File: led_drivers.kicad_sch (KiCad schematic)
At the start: 23 parts, among them IC1 SamacSys_Parts_HT16K33-28SOP, IC2 SamacSys_Parts_HT16K33-28SOP, SW1 SW_Omron_B3FS, SW2 SW_Omron_B3FS, SW3 SW_Omron_B3FS, SW4 SW_Omron_B3FS

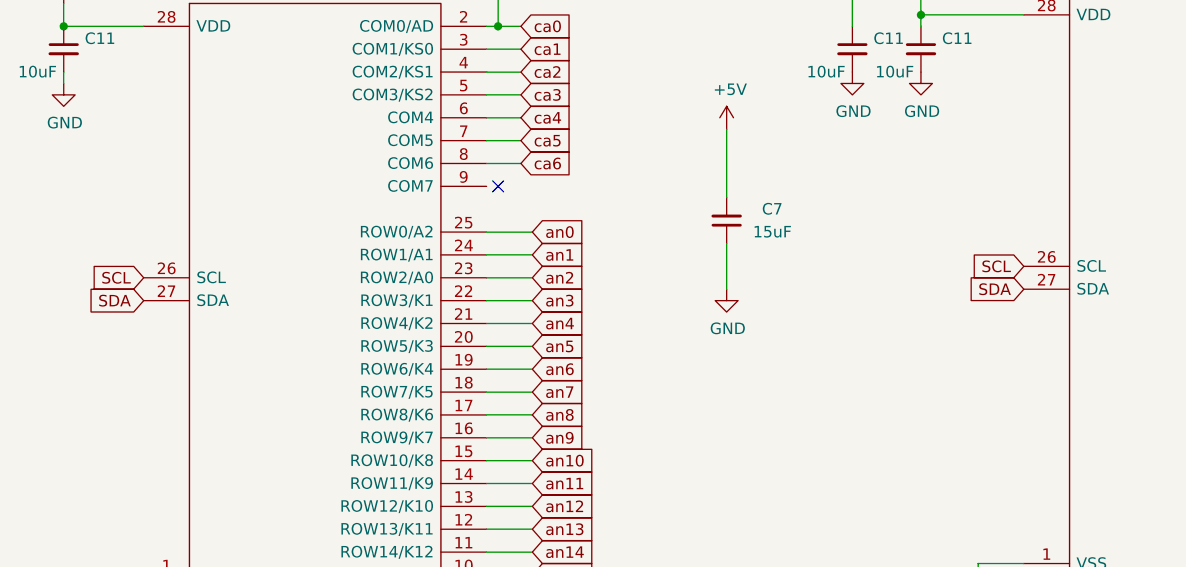
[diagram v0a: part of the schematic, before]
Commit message: Add i2c transciever, Pitanga V2
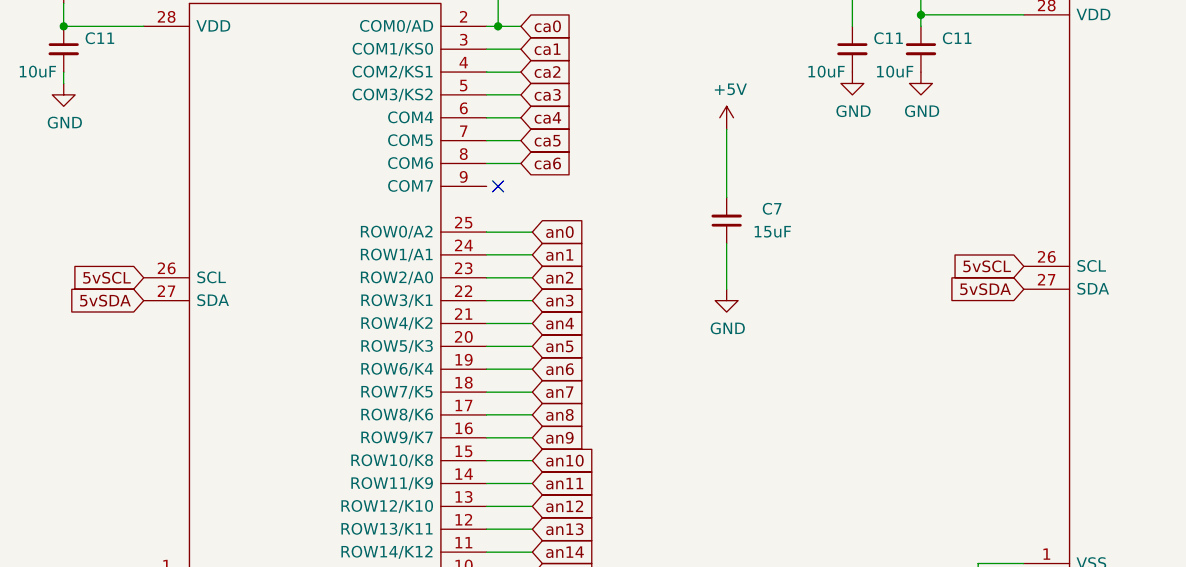
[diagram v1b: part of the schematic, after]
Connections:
- net SCL renamed 5vSCL
- net SDA renamed 5vSDA
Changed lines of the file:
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@@
     (stroke (width 0) (type default))
   )
-  (global_label "SCL" (shape input) (at 54.61 81.28 180)
+  (global_label "5vSCL" (shape input) (at 54.61 81.28 180)
     (effects (font (size 1.27 1.27)) (justify right))
     (property "Intersheetrefs" "${INTERSHEET_REFS}" (at 48.1966 81.28 0)
@@
     )
   )
-  (global_label "SCL" (shape input) (at 152.4 80.01 180)
+  (global_label "5vSCL" (shape input) (at 152.4 80.01 180)
     (effects (font (size 1.27 1.27)) (justify right))
     (property "Intersheetrefs" "${INTERSHEET_REFS}" (at 145.9866 80.01 0)
@@
     )
   )
-  (global_label "SDA" (shape input) (at 54.61 83.82 180)
+  (global_label "5vSDA" (shape input) (at 54.61 83.82 180)
     (effects (font (size 1.27 1.27)) (justify right))
     (property "Intersheetrefs" "${INTERSHEET_REFS}" (at 54.61 83.82 0)
@@
     )
   )
-  (global_label "SDA" (shape input) (at 152.4 82.55 180)
+  (global_label "5vSDA" (shape input) (at 152.4 82.55 180)
     (effects (font (size 1.27 1.27)) (justify right))
     (property "Intersheetrefs" "${INTERSHEET_REFS}" (at 152.4 82.55 0)
